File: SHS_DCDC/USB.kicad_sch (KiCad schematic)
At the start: 24 parts, among them J2 USB_A, Q8 Q_PMOS_DGS, U4 LMV358IDR, U5 MP3414A

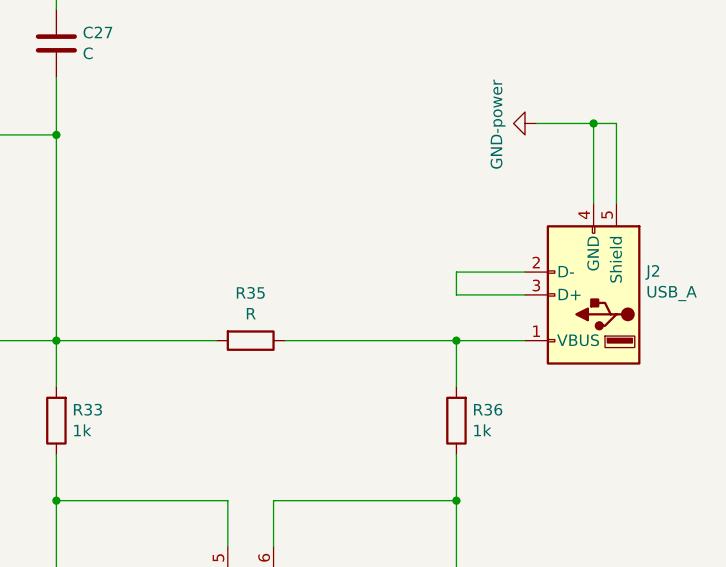
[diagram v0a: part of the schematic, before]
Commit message: Ubuntu transfer
Commit before transfer onto Ubuntu
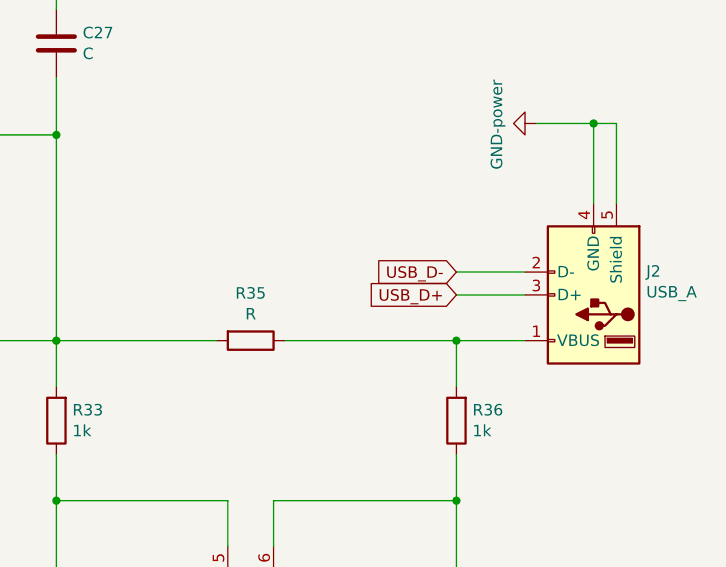
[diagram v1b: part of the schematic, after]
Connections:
- net USB_D+: now reaches J2.3 (D+)
- net USB_D+: no longer J2.2 (D-)
- new net USB_D-: J2.2 (D-)
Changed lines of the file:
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@@
-    (stroke (width 0) (type default) (color 0 0 0 0))
-  )
-  (wire (pts (xy 236.22 67.31) (xy 236.22 64.77))
     (stroke (width 0) (type default) (color 0 0 0 0))
   )
@@
     )
   )
+  (global_label "USB_D+" (shape input) (at 236.22 67.31 180) (fields_autoplaced)
+    (effects (font (size 1.27 1.27)) (justify right))
+    (property "Intersheet References" "${INTERSHEET_REFS}" (id 0) (at 226.2758 67.2306 0)
+      (effects (font (size 1.27 1.27)) (justify right) hide)
+    )
+  )
   (global_label "ILIM_USB" (shape input) (at 80.01 102.87 270) (fields_autoplaced)
     (effects (font (size 1.27 1.27)) (justify right))
@@
     )
   )
+  (global_label "USB_D-" (shape input) (at 236.22 64.77 180) (fields_autoplaced)
+    (effects (font (size 1.27 1.27)) (justify right))
+    (property "Intersheet References" "${INTERSHEET_REFS}" (id 0) (at 226.2758 64.6906 0)
+      (effects (font (size 1.27 1.27)) (justify right) hide)
+    )
+  )
